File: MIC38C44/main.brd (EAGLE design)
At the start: 137.1 x 162.2 mm, 59 parts, among them Q1 800-1000V

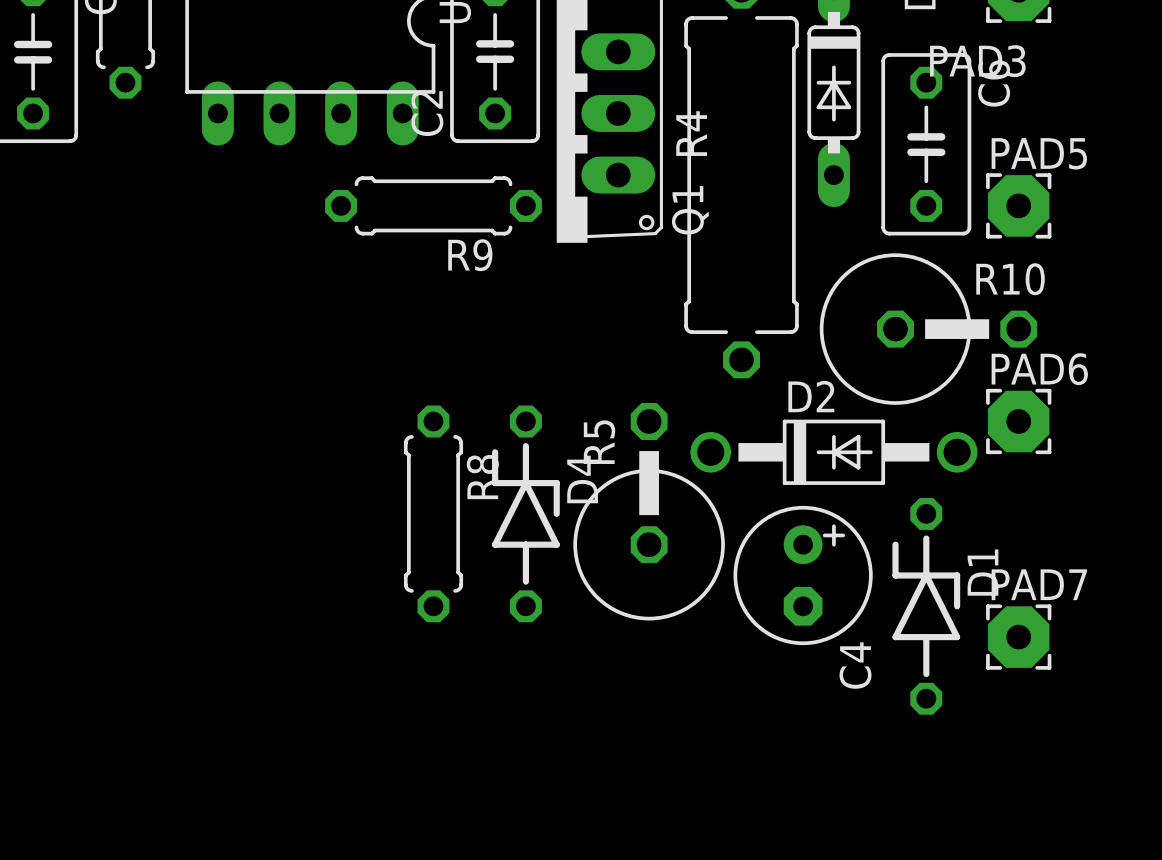
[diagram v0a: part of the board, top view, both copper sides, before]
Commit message: -a
a
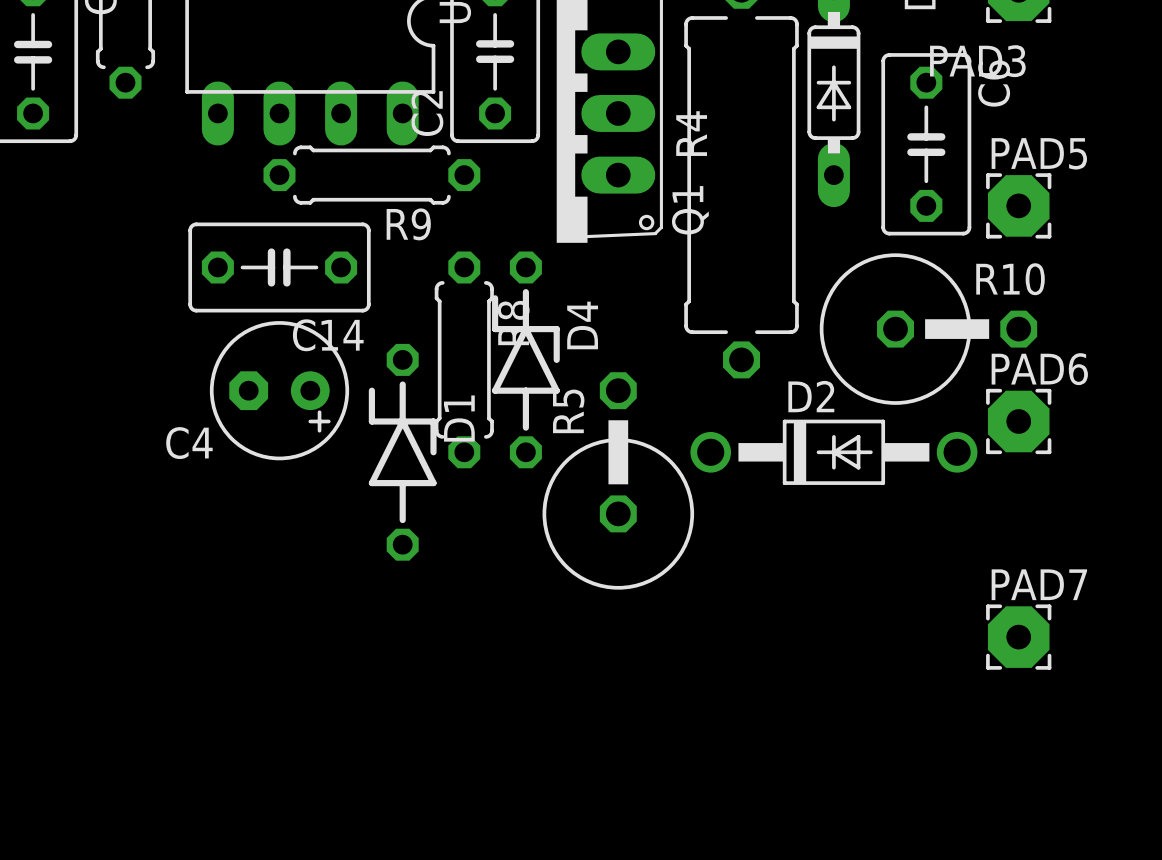
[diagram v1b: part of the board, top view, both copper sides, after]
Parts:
- added C14: 100n, rcl:C050-035X075
- D1, D4: value 18 -> 18V
- moved C4 22.9 mm to (22.9, 22.9), turned to 180 degrees
- moved D1 22.5 mm to (27.9, 20.3)
- moved R8 6.48 mm to (30.5, 24.1)
- moved D4 6.35 mm to (33.0, 24.1)
- moved R9 2.84 mm to (26.7, 31.8)
- moved R5 1.80 mm to (36.8, 20.3)
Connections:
- net GND: now also C14.2
- net N$11: now also R5.1; no longer R5.2
- net VDD: now also C14.1, R5.2; no longer R5.1
